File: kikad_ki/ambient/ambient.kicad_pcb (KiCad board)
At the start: 2 copper layers, 80 x 66 mm, 69 parts, among them J1 5V DC, J2 FPC 01x10 Female, J3 LED Array, Q1 2N3904, SW1 Reset, SW2 Next, SW3 Select, SW4 Modify, U1 ATmega328P-PU, U2 AT24C256, U3 AT24C256, U4 AT24C256, U5 AT24C256, Y1 16 MHz

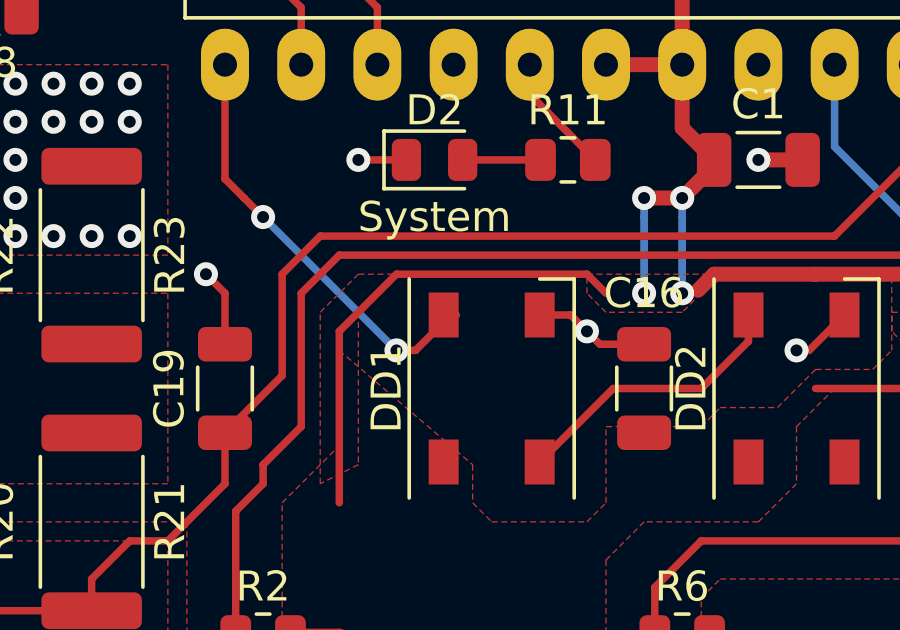
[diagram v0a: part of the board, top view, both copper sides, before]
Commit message: changes
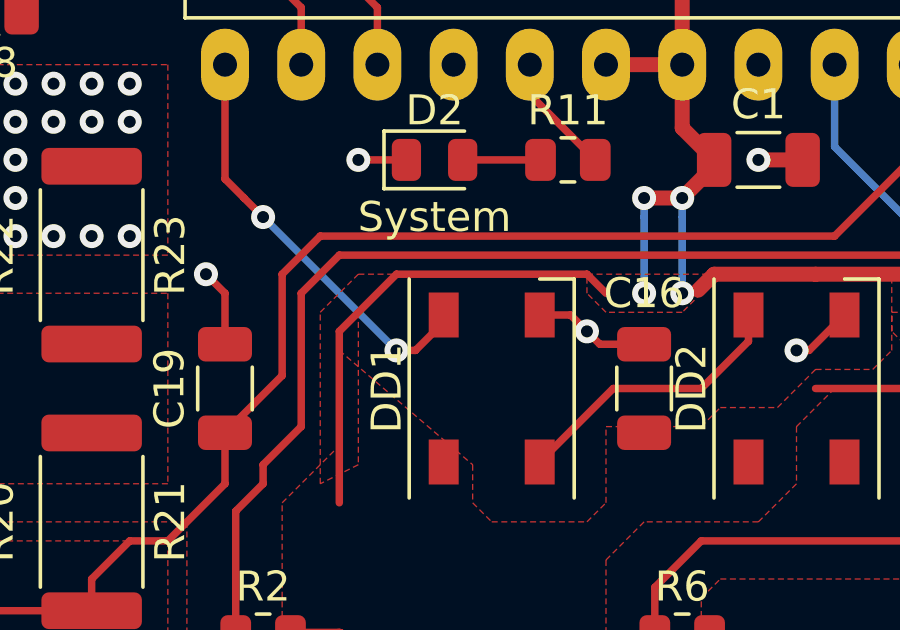
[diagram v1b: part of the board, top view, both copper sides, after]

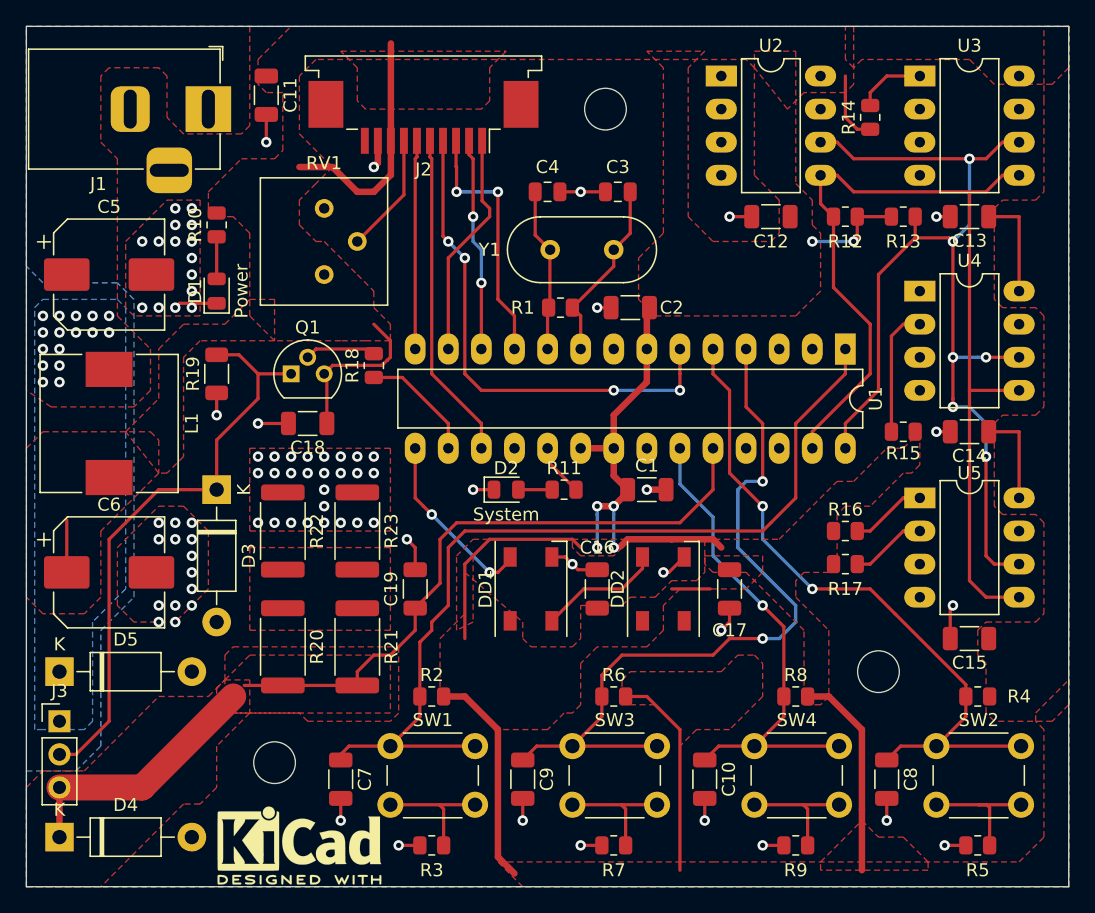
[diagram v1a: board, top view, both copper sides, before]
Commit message: fixes
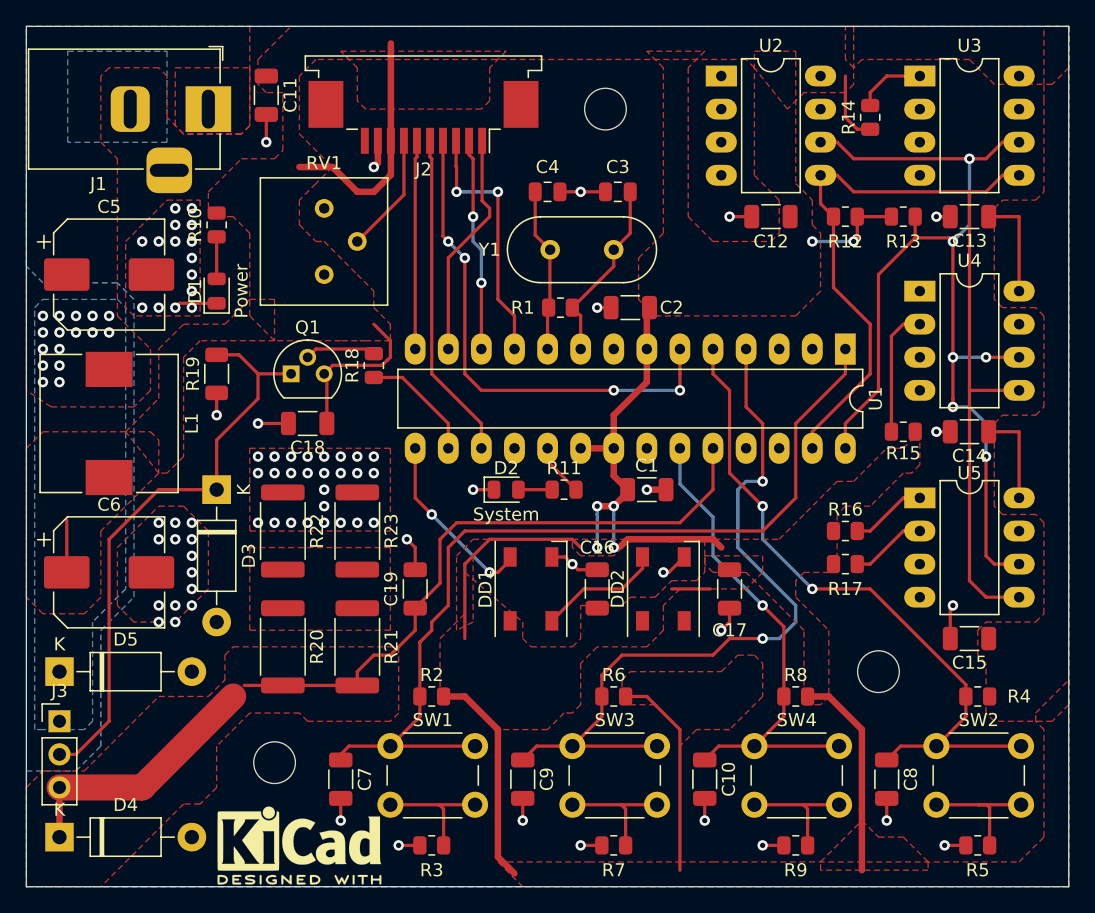
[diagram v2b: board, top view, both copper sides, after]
